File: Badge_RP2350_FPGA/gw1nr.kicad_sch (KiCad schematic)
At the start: 24 parts, among them U2 GW1N-LV9QN88C6_I5_, U6 W25Q32JVSS

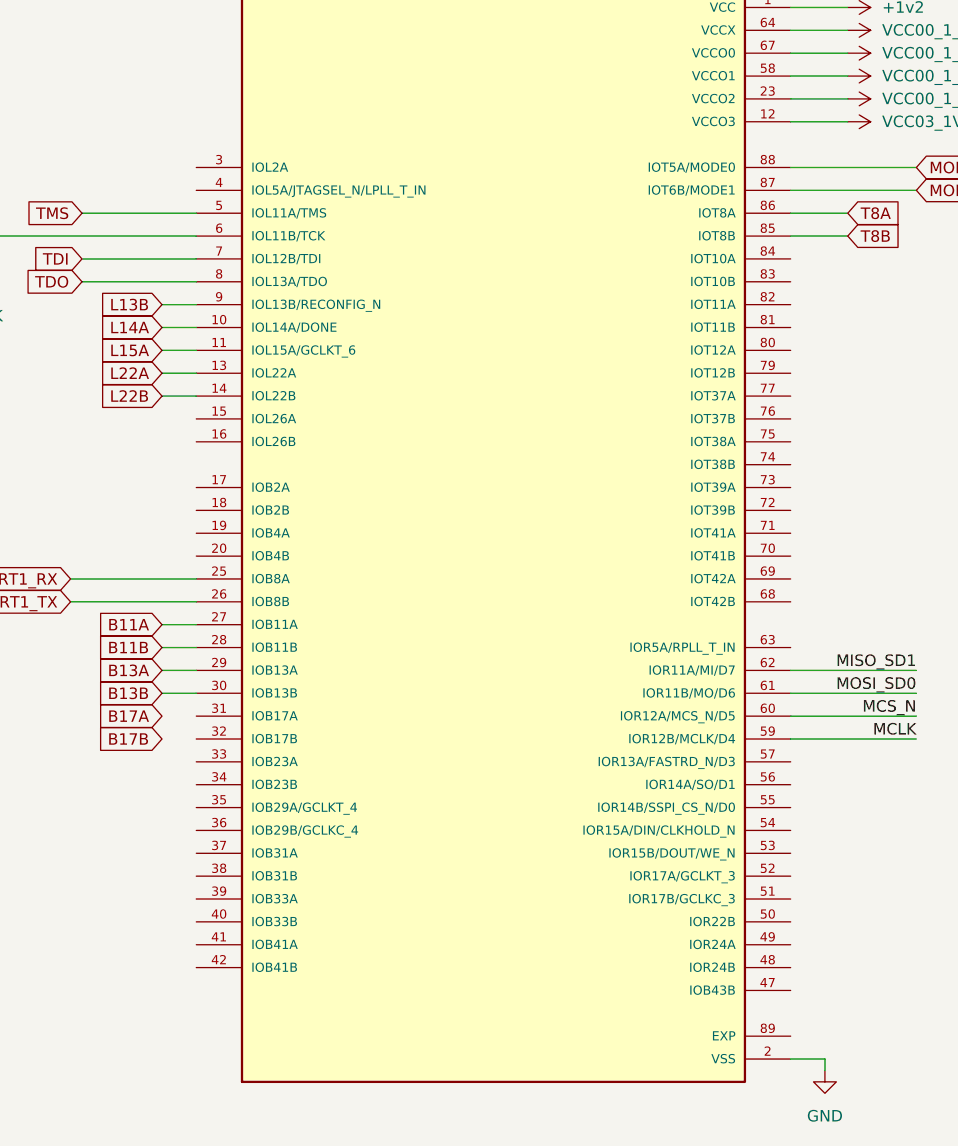
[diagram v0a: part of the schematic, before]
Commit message: add x to unused pins and connect more pins
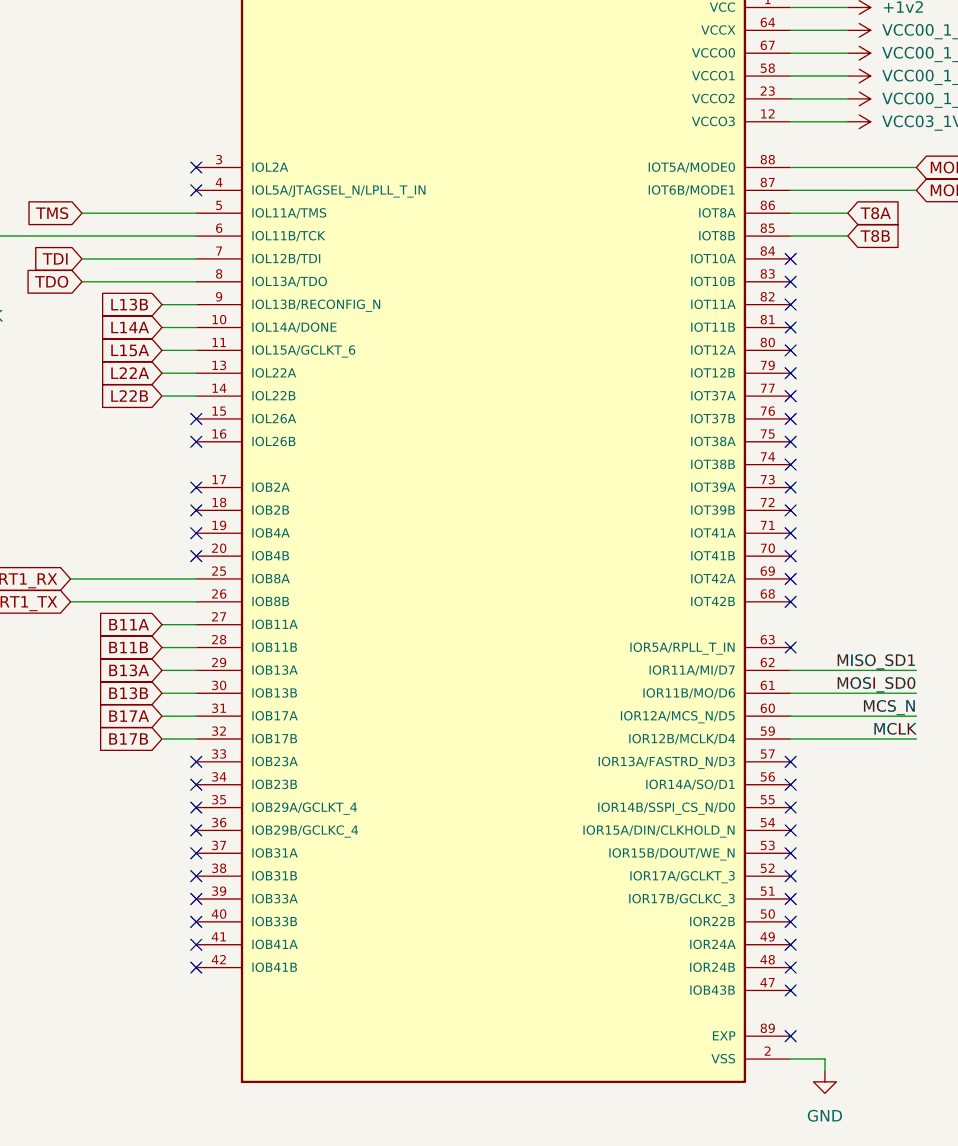
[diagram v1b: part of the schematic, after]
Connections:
- net B17A: now also U2.31 (IOB17A)
- net B17B: now also U2.32 (IOB17B)
- no-connect marks 2 -> 49
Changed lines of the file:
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@@
+	)
+	(no_connect
+		(at 138.43 135.89)
+	)
+	(no_connect
+		(at 138.43 72.39)
+	)
+	(no_connect
+		(at 138.43 130.81)
+	)
+	(no_connect
+		(at 138.43 82.55)
+	)
+	(no_connect
+		(at 138.43 151.13)
+	)
+	(no_connect
+		(at 72.39 59.69)
+	)
+	(no_connect
+		(at 138.43 85.09)
+	)
+	(no_connect
+		(at 138.43 156.21)
+	)
+	(no_connect
+		(at 138.43 100.33)
+	)
+	(no_connect
+		(at 72.39 90.17)
+	)
+	(no_connect
+		(at 138.43 125.73)
+	)
+	(no_connect
+		(at 72.39 135.89)
+	)
+	(no_connect
+		(at 72.39 125.73)
+	)
+	(no_connect
+		(at 138.43 133.35)
+	)
+	(no_connect
+		(at 138.43 92.71)
+	)
+	(no_connect
+		(at 72.39 102.87)
+	)
+	(no_connect
+		(at 138.43 80.01)
+	)
+	(no_connect
+		(at 138.43 102.87)
+	)
+	(no_connect
+		(at 72.39 97.79)
+	)
+	(no_connect
+		(at 72.39 146.05)
+	)
+	(no_connect
+		(at 72.39 140.97)
 	)
 	(no_connect
@@
 	)
 	(no_connect
+		(at 138.43 128.27)
+	)
+	(no_connect
 		(at 234.95 134.62)
 	)
+	(no_connect
+		(at 72.39 128.27)
+	)
+	(no_connect
+		(at 72.39 95.25)
+	)
+	(no_connect
+		(at 72.39 87.63)
+	)
+	(no_connect
+		(at 72.39 62.23)
+	)
+	(no_connect
+		(at 138.43 107.95)
+	)
+	(no_connect
+		(at 138.43 87.63)
+	)
+	(no_connect
+		(at 72.39 133.35)
+	)
+	(no_connect
+		(at 72.39 130.81)
+	)
+	(no_connect
+		(at 138.43 77.47)
+	)
+	(no_connect
+		(at 138.43 148.59)
+	)
+	(no_connect
+		(at 138.43 95.25)
+	)
+	(no_connect
+		(at 72.39 148.59)
+	)
+	(no_connect
+		(at 138.43 90.17)
+	)
+	(no_connect
+		(at 138.43 97.79)
+	)
+	(no_connect
+		(at 72.39 138.43)
+	)
+	(no_connect
+		(at 138.43 138.43)
+	)
+	(no_connect
+		(at 138.43 113.03)
+	)
+	(no_connect
+		(at 138.43 143.51)
+	)
+	(no_connect
+		(at 138.43 146.05)
+	)
+	(no_connect
+		(at 138.43 140.97)
+	)
+	(no_connect
+		(at 138.43 74.93)
+	)
+	(no_connect
+		(at 138.43 105.41)
+	)
+	(no_connect
+		(at 72.39 100.33)
+	)
+	(no_connect
+		(at 72.39 143.51)
+	)
+	(no_connect
+		(at 138.43 69.85)
+	)
+	(wire
+		(pts
+			(xy 68.58 123.19) (xy 72.39 123.19)
+		)
+		(stroke
+			(width 0)
+			(type default)
+		)
+	)
 	(wire
 		(pts
@@
 		)
 		(stroke
+			(width 0)
+			(type default)
+		)
+	)
+	(wire
+		(pts
+			(xy 68.58 120.65) (xy 72.39 120.65)
+		)
+		(stroke
